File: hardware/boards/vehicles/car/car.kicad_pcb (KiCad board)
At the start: 2 copper layers, 50 x 95 mm, 119 parts, among them J1 Conn_01x04_Socket, J10 Conn_02x03_Odd_Even, J2 Conn_01x05_Socket, J3 Conn_01x05_Socket, J4 Conn_01x05_Socket, J5 Conn_01x02_Socket, J6 SMA, J7 02x04, J8 Conn_01x04_Socket, J9 Conn_02x05_Odd_Even, M1 Motor_DC, M2 Motor_DC, Q1 FQP27P06, Q10 AO3400A, Q11 2N3904, Q12 2N3904, Q2 AO3400A, Q3 FQP27P06, Q4 AO3400A, Q5 2N3904, Q6 2N3904, Q7 FQP27P06, Q8 AO3400A, Q9 FQP27P06, SW1 SW_Push, U1 ATmega328P-A, U4 TPS54302, U5 AMS1117-3.3, U7 NRF24L01, U8 RFX2401C, Y1 8MHz, Y3 16MHz

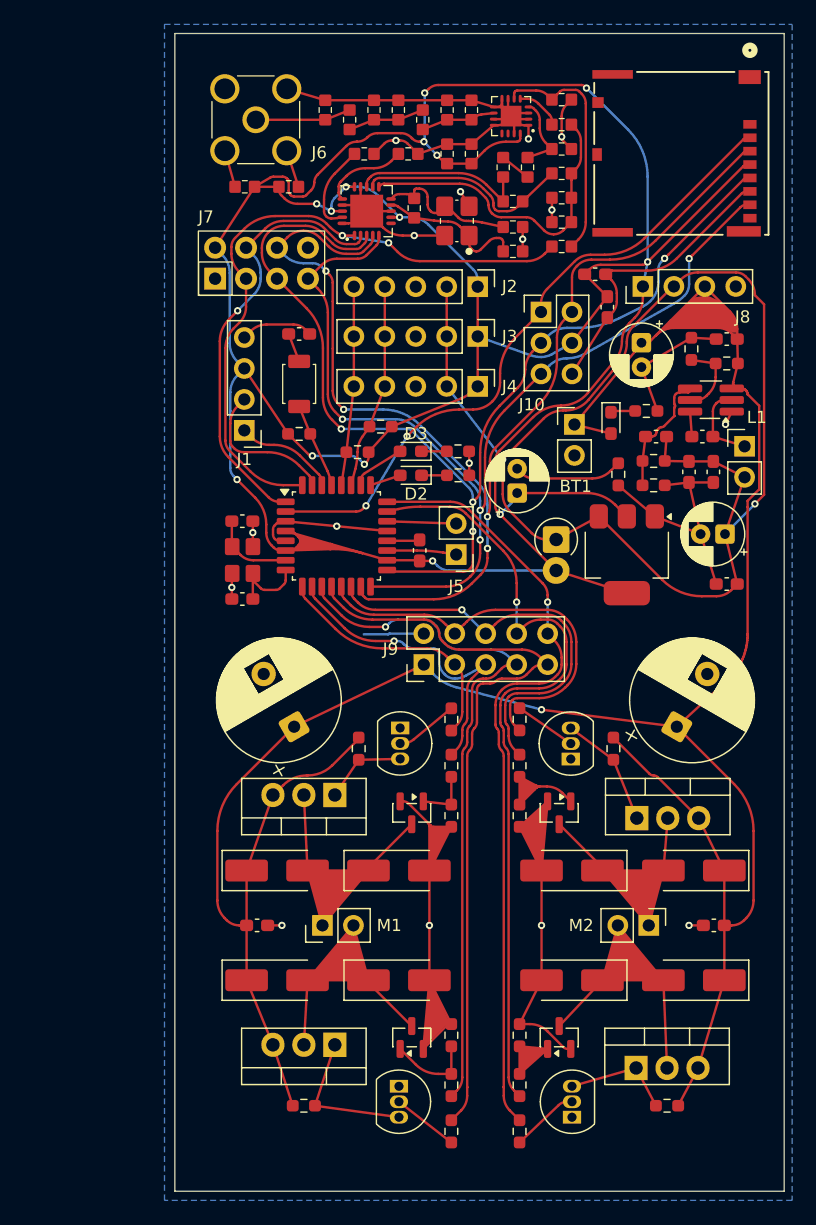
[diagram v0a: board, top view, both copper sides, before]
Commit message: REFACTO relinked every kicad projects
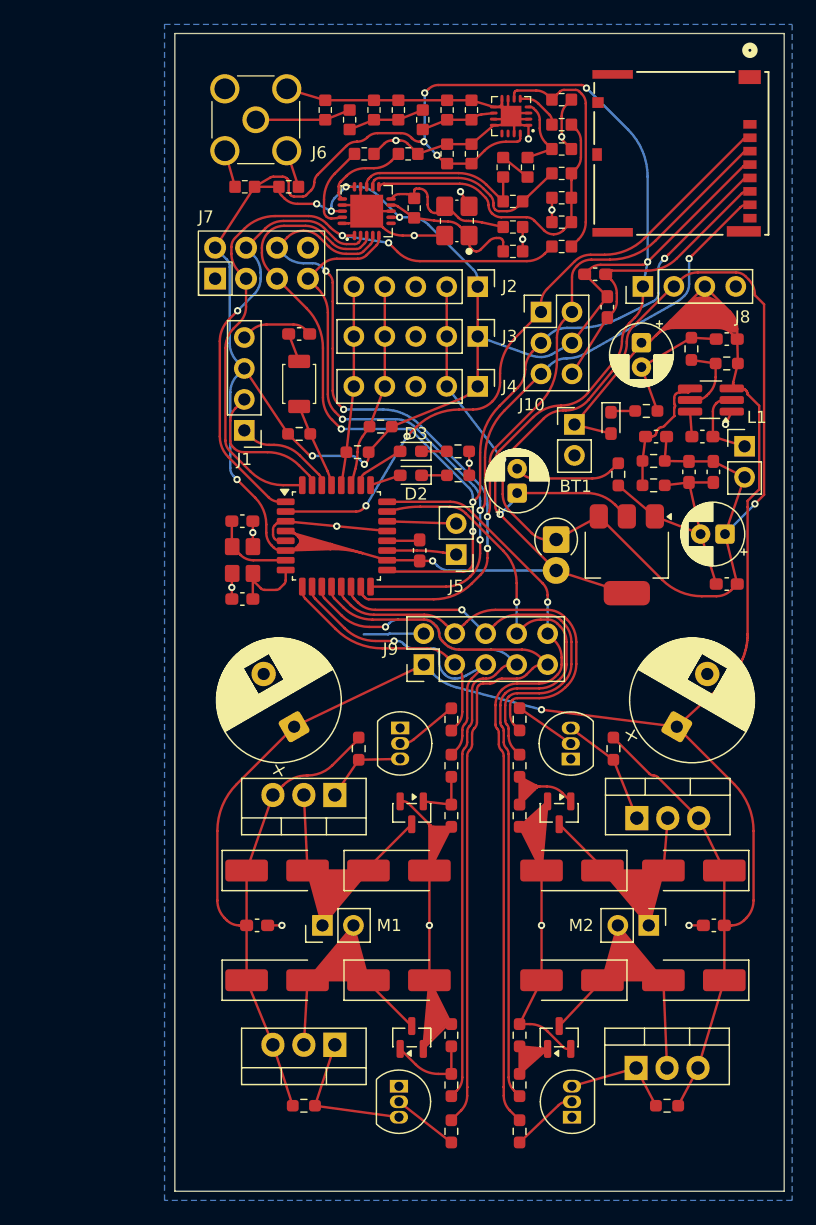
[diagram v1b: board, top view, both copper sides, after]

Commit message: car PCB
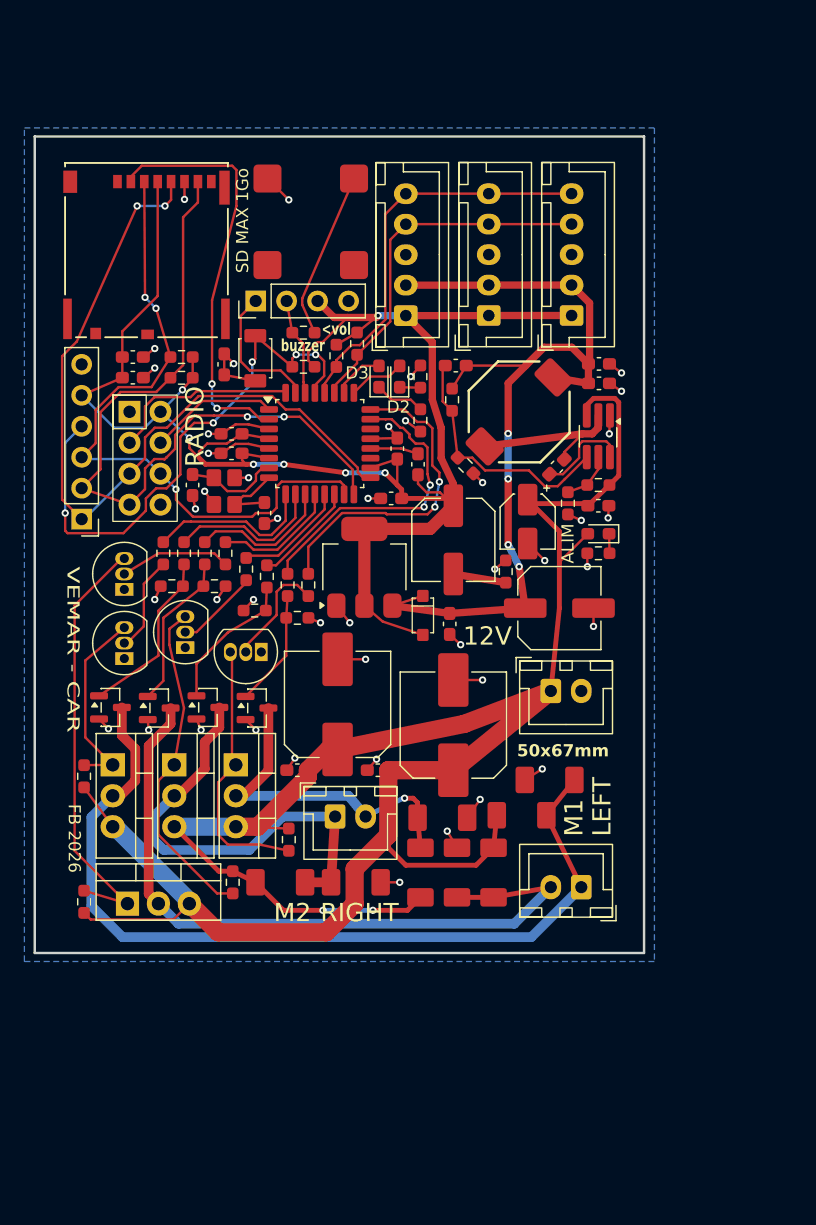
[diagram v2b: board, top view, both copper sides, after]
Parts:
- removed C24: 75pF, Capacitor_SMD:C_0603_1608Metric_Pad1.08x0.95mm_HandSolder
- removed C25: 10nF, common:C_0603
- removed C26: 1nF, common:C_0603
- removed C27: 33nF, common:C_0603
- removed C28, C29: 12pF, common:C_0603
- removed C30: 2.2nF, common:C_0603
- removed C31: 4.7nF, common:C_0603
- removed C32, C37, C38, C39, C40: 1.5pF, common:C_0603
- removed C33: 1.0pF, common:C_0603
- removed C34: 220pF, common:C_0603
- removed C35: 1uF, common:C_0603
- removed C36: 0.3pF, common:C_0603
- removed C41, C43: 22uF, Capacitor_THT:CP_Radial_D5.0mm_P2.00mm
- removed C42: 100nF, Capacitor_SMD:C_0603_1608Metric_Pad1.08x0.95mm_HandSolder
- removed J10: Conn_02x03_Odd_Even, Connector_PinHeader_2.54mm:PinHeader_2x03_P2.54mm_Vertical
- removed J7: 02x04, connector:Pin_02x04
- removed J8: Conn_01x04_Socket, Connector_PinHeader_2.54mm:PinHeader_1x04_P2.54mm_Vertical
- removed J9: Conn_02x05_Odd_Even, Connector_PinHeader_2.54mm:PinHeader_2x05_P2.54mm_Vertical
- removed L10, L9: 2.4nH, common:L_0603
- removed L6: 8.2nH, common:L_0603
- removed L7: 2.7nH, common:L_0603
- removed L8: 3.9nH, common:L_0603
- removed R31: 1, Resistor_SMD:R_0603_1608Metric_Pad0.98x0.95mm_HandSolder
- removed R32: 1M, common:R_0603
- removed U4: TPS54302, Package_TO_SOT_SMD:TSOT-23-6_HandSoldering
- removed U5: AMS1117-3.3, Package_TO_SOT_SMD:SOT-223-3_TabPin2
- removed U7: NRF24L01, transceiver:NRF24L01_QFN20
- removed U8: RFX2401C, transceiver:RFX2401C_QFN16
- removed Y3: 16MHz, common:Crystal_3225
- added BZ1: Buzzer, common:buzzer_8.5x8.5, F.Cu at (135.5, 69.7)
- added C10: 100nF, Capacitor_SMD:C_0603_1608Metric_Pad1.08x0.95mm_HandSolder, F.Cu at (159.1, 93.0)
- added C11: 100nF, Capacitor_SMD:C_0603_1608Metric_Pad1.08x0.95mm_HandSolder, F.Cu at (155.7, 89.8)
- added C12: 22uF, Capacitor_SMD:C_0603_1608Metric_Pad1.08x0.95mm_HandSolder, F.Cu at (159.2, 83.0)
- added C17: 22uF, common:CP_Elec_6.3x5.4, F.Cu at (147.2, 95.8)
- added C18: 100nF, Capacitor_SMD:C_0603_1608Metric_Pad1.08x0.95mm_HandSolder, F.Cu at (120.9, 82.5)
- added C7: 100nF, Capacitor_SMD:C_0603_1608Metric_Pad1.08x0.95mm_HandSolder, F.Cu at (142.6, 88.3)
- added C8: 100nF, Capacitor_SMD:C_0603_1608Metric_Pad1.08x0.95mm_HandSolder, F.Cu at (144.3, 89.6)
- added C9: 10uF, Capacitor_SMD:CP_Elec_4x5.4, F.Cu at (153.3, 94.3)
- added U2: TPS54302, Package_TO_SOT_SMD:TSOT-23-6_HandSoldering, F.Cu at (159.1, 87.3)
- added U3: AMS1117-3.3, Package_TO_SOT_SMD:SOT-223-3_TabPin2, F.Cu at (139.9, 98.0)
- BT1: value Battery 12V -> JST; footprint Connector_PinHeader_2.54mm:PinHeader_1x02_P2.54mm_Vertical -> Connector_JST:JST_XH_B2B-XH-A_1x02_P2.50mm_Vertical
- C13: value 470uF -> 22uF; footprint Capacitor_THT:CP_Radial_D10.0mm_P5.00mm -> Capacitor_SMD:C_0603_1608Metric_Pad1.08x0.95mm_HandSolder
- C14: value 100nF -> 75pF
- C15: value 470uF -> 22uF; footprint Capacitor_THT:CP_Radial_D10.0mm_P5.00mm -> common:CP_Elec_6.3x5.4
- C19: footprint Capacitor_THT:CP_Radial_D5.0mm_P2.00mm -> Capacitor_SMD:C_0603_1608Metric_Pad1.08x0.95mm_HandSolder
- C20: value 100nF -> 470uF; footprint Capacitor_SMD:C_0603_1608Metric_Pad1.08x0.95mm_HandSolder -> common:CP_Elec_8x10.5
- C22: value 22uF -> 470uF; footprint Capacitor_SMD:C_0603_1608Metric_Pad1.08x0.95mm_HandSolder -> common:CP_Elec_8x10.5
- C23: value 22uF -> 100nF
- C4: value 100nF -> 4.7uF
- C5: value 10uF -> 100nF
- D1, D3: value LED -> RED
- D10, D11, D5, D6, D7, D8, D9: footprint Diode_SMD:D_SMA_Handsoldering -> common:SMA(DO-214AC)
- D12: value 1N400x -> SS36; footprint Diode_THT:D_DO-41_SOD81_P2.54mm_Vertical_AnodeUp -> common:SMA(DO-214AC)
- D2: value LED -> GREEN
- D4: value SS36 -> RS1MFA; footprint Diode_SMD:D_SMA_Handsoldering -> common:D_SOD123
- J1: value Conn_01x04_Socket -> Dupont; footprint Connector_PinHeader_2.54mm:PinHeader_1x04_P2.54mm_Vertical -> Connector_PinHeader_2.54mm:PinHeader_1x06_P2.54mm_Vertical
- J2: value Conn_01x05_Socket -> Dupont; footprint Connector_PinHeader_2.54mm:PinHeader_1x05_P2.54mm_Vertical -> Connector_PinHeader_2.54mm:PinHeader_1x04_P2.54mm_Vertical
- J3: value Conn_01x05_Socket -> Dupont; footprint Connector_PinHeader_2.54mm:PinHeader_1x05_P2.54mm_Vertical -> connector:Pin_02x04
- J4: value Conn_01x05_Socket -> JST; footprint Connector_PinHeader_2.54mm:PinHeader_1x05_P2.54mm_Vertical -> Connector_JST:JST_XH_B5B-XH-A_1x05_P2.50mm_Vertical
- J5: value Conn_01x02_Socket -> JST; footprint Connector_PinHeader_2.54mm:PinHeader_1x02_P2.54mm_Vertical -> Connector_JST:JST_XH_B5B-XH-A_1x05_P2.50mm_Vertical
- J6: value SMA -> JST; footprint connector:SMA -> Connector_JST:JST_XH_B5B-XH-A_1x05_P2.50mm_Vertical
- L1: footprint Connector_PinHeader_2.54mm:PinHeader_1x02_P2.54mm_Vertical -> common:Inductor_octogone
- M1: value Motor_DC -> LEFT; footprint Connector_PinHeader_2.54mm:PinHeader_1x02_P2.54mm_Vertical -> Connector_JST:JST_XH_B2B-XH-A_1x02_P2.50mm_Vertical
- M2: value Motor_DC -> RIGHT; footprint Connector_PinHeader_2.54mm:PinHeader_1x02_P2.54mm_Vertical -> Connector_JST:JST_XH_B2B-XH-A_1x02_P2.50mm_Vertical
- Q2, Q8: value AO3400A -> FQP27P06; footprint Package_TO_SOT_SMD:SOT-23 -> Package_TO_SOT_THT:TO-220-3_Vertical
- Q3, Q9: value FQP27P06 -> AO3400A; footprint Package_TO_SOT_THT:TO-220-3_Vertical -> Package_TO_SOT_SMD:SOT-23
- R10: value 10K -> 43.2K
- R11: value 10K -> 5.76K
- R12: value 4.7K -> 1
- R13, R21: value 47 -> 10K
- R14, R22: value 1K -> 10K
- R16: value 47 -> 1K
- R17: value 4.7K -> 47
- R18: value 10K -> 47
- R19: value 10K -> 4.7K
- R23: value 511K -> 1K
- R24: value 22k -> 1K; footprint common:R_0603 -> Resistor_SMD:R_0603_1608Metric_Pad0.98x0.95mm_HandSolder
- R25: value 105K -> 47
- R26: value 1k -> 47; footprint common:R_0603 -> Resistor_SMD:R_0603_1608Metric_Pad0.98x0.95mm_HandSolder
- R27: value 1k -> 4.7K; footprint common:R_0603 -> Resistor_SMD:R_0603_1608Metric_Pad0.98x0.95mm_HandSolder
- R28: value 20k -> 4.7K; footprint common:R_0603 -> Resistor_SMD:R_0603_1608Metric_Pad0.98x0.95mm_HandSolder
- R29: value 43.2K -> 10K
- R30: value 5.76K -> 10K
- R5: value 4.7K -> ?
- R7: value 1K -> 4.7K
- R8: value 47 -> 511K
- R9: value 4.7K -> 105K
- SD1: value ~ -> SD Card Slot
- Y1: value 8MHz -> 16MHz
- moved R14 65.7 mm to (124.9, 82.5), turned to 180 degrees
- moved R28 64.7 mm to (133.7, 120.4), turned to -90 degrees
- moved R13 63.7 mm to (124.9, 80.8), turned to 180 degrees
- moved R27 58.7 mm to (129.1, 123.9), turned to 90 degrees
- moved R22 51.3 mm to (127.6, 99.6), turned to 180 degrees
- moved R20 50.7 mm to (116.9, 125.5), turned to 90 degrees
- moved R21 49.9 mm to (124.1, 99.6), turned to 180 degrees
- moved C14 48.7 mm to (147.4, 81.5)
- moved R12 46.9 mm to (151.5, 98.4), turned to -90 degrees
- moved R11 46.8 mm to (148.2, 89.7), turned to 135 degrees
- moved Q6 46.6 mm to (120.2, 99.9), turned to 90 degrees
- moved Q9 45.9 mm to (127.1, 109.5)
- moved Q12 45.9 mm to (131.4, 105.0), turned to 180 degrees
- moved SD1 44.6 mm to (122.0, 72.0), turned to 0 degrees
- moved R26 44.0 mm to (133.6, 99.5), turned to 90 degrees
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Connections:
- C1 pad 2: Net-(C1-Pad2) -> GND
- C13 pad 1: 12V -> GND
- C13 pad 2: GND -> 5V
- C14 pad 1: 12V -> Net-(U2-FB)
- C14 pad 2: GND -> 5V
- C15 pad 1: 12V -> 5V
- C16 pad 1: 12V -> GND
- C16 pad 2: GND -> 5V
- C19 pad 1: 12V -> 3V3
- C20 pad 1: GND -> 12V
- C20 pad 2: 12V -> GND
- C21 pad 1: Net-(U4-BOOT) -> 12V
- C21 pad 2: Net-(U4-SW) -> GND
- C22 pad 1: 5V -> 12V
- C23 pad 1: GND -> 12V
- C23 pad 2: 5V -> GND
- C4 pad 2: Net-(U1-AREF) -> GND
- D10 pad 1: 12V -> Net-(D10-K)
- D10 pad 2: Net-(D10-A) -> GND
- D11 pad 1: Net-(D10-A) -> 12V
- D11 pad 2: GND -> Net-(D11-A)
- D12 pad 1: 5V -> Net-(D11-A)
- D12 pad 2: 3V3 -> GND
- D4 pad 1: 12V -> 5V
- D4 pad 2: Net-(D4-A) -> 3V3
- D5 pad 1: Net-(D4-A) -> 12V
- D5 pad 2: GND -> Net-(D5-A)
- D6 pad 1: 12V -> Net-(D5-A)
- D6 pad 2: Net-(D6-A) -> GND
- D7 pad 1: Net-(D6-A) -> 12V
- D7 pad 2: GND -> Net-(D7-A)
- D8 pad 1: 12V -> Net-(D7-A)
- D8 pad 2: Net-(D8-A) -> GND
- D9 pad 1: Net-(D8-A) -> 12V
- D9 pad 2: GND -> Net-(D10-K)
- J1 pad 1: RX -> SCK
- J1 pad 2: TX -> MISO
- J1 pad 3: 3V3 -> MOSI
- J1 pad 4: GND -> RST
- J2 pad 1: 3V3 -> TX
- J2 pad 2: 5V -> RX
- J2 pad 3: GND -> 3V3
- J2 pad 4: SDA -> GND
- J3 pad 1: 3V3 -> GND
- J3 pad 2: 5V -> RC_EN
- J3 pad 3: GND -> SCK
- J3 pad 4: SDA -> MISO
- J3 pad 5: SCL -> unconnected-(J3-Pad5)
- J5 pad 1: ADC0 -> 3V3
- J5 pad 2: ADC1 -> 5V
- J6 pad 1: Net-(J6-ANT) -> 3V3
- J6 pad 2: GND -> 5V
- J6 pad 4: GND -> SDA
- J6 pad 5: GND -> SCL
- L1 pad 1: Net-(U4-SW) -> Net-(U2-SW)
- M1 pad 1: Net-(D4-A) -> Net-(D5-A)
- M1 pad 2: Net-(D6-A) -> Net-(D7-A)
- M2 pad 1: Net-(D8-A) -> Net-(D10-K)
- M2 pad 2: Net-(D10-A) -> Net-(D11-A)
- Q1 pad 2: Net-(D4-A) -> Net-(D5-A)
- Q10 pad 3: Net-(D10-A) -> Net-(D11-A)
- Q2 pad 2: GND -> Net-(D7-A)
- Q2 pad 3: Net-(D4-A) -> 12V
- Q3 pad 2: Net-(D6-A) -> GND
- Q3 pad 3: 12V -> Net-(D5-A)
- Q4 pad 3: Net-(D6-A) -> Net-(D7-A)
- Q6 pad 3: Net-(Q3-G) -> Net-(Q2-G)
- Q7 pad 2: Net-(D8-A) -> Net-(D10-K)
- Q8 pad 1: Net-(Q8-G) -> Net-(Q12-C)
- Q8 pad 2: GND -> Net-(D11-A)
- Q8 pad 3: Net-(D8-A) -> 12V
- Q9 pad 1: Net-(Q12-C) -> Net-(Q9-G)
- Q9 pad 2: Net-(D10-A) -> GND
- Q9 pad 3: 12V -> Net-(D10-K)
- R10 pad 1: Net-(Q2-G) -> Net-(U2-FB)
- R10 pad 2: GND -> 5V
- R11 pad 2: Net-(Q4-G) -> Net-(U2-FB)
- R12 pad 1: 12V -> GND
- R12 pad 2: Net-(Q3-G) -> Net-(C17-Pad2)
- R13 pad 1: Net-(Q4-G) -> 3V3
- R13 pad 2: M1_EN_CW -> MOSI
- R14 pad 1: M1_EN_CCW -> 3V3
- R14 pad 2: Net-(Q6-B) -> MISO
- R15 pad 1: M2_PWM_CW -> M1_PWM_CW
- R15 pad 2: Net-(Q11-B) -> Net-(Q5-B)
- R16 pad 1: Net-(Q8-G) -> M1_EN_CCW
- R16 pad 2: M2_PWM_CCW -> Net-(Q6-B)
- R17 pad 1: Net-(Q11-C) -> Net-(Q3-G)
- R17 pad 2: 12V -> M1_PWM_CCW
- R18 pad 1: Net-(Q8-G) -> Net-(Q4-G)
- R18 pad 2: GND -> M1_EN_CW
- R19 pad 1: GND -> Net-(Q1-G)
- R19 pad 2: Net-(Q10-G) -> 12V
- R20 pad 2: Net-(Q12-C) -> Net-(Q2-G)
- R21 pad 1: Net-(Q10-G) -> Net-(Q3-G)
- R21 pad 2: M2_EN_CW -> GND
- R22 pad 1: M2_EN_CCW -> GND
- R22 pad 2: Net-(Q12-B) -> Net-(Q4-G)
- R23 pad 1: Net-(U4-EN) -> M2_PWM_CW
- R23 pad 2: 12V -> Net-(Q11-B)
- R24 pad 1: GND -> M2_EN_CCW
- R24 pad 2: Net-(U7-IREF) -> Net-(Q12-B)
- R25 pad 1: GND -> Net-(Q9-G)
- R25 pad 2: Net-(U4-EN) -> M2_PWM_CCW
- R26 pad 1: Net-(U7-VDD_PA) -> Net-(Q10-G)
- R26 pad 2: Net-(U8-TXEN) -> M2_EN_CW
- R27 pad 1: RC_EN -> Net-(Q11-C)
- R27 pad 2: Net-(U8-RXEN) -> 12V
- R28 pad 1: GND -> 12V
- R28 pad 2: Net-(U8-RXEN) -> Net-(Q12-C)
- R29 pad 1: Net-(U4-FB) -> Net-(Q9-G)
- R29 pad 2: 5V -> GND
- R30 pad 2: Net-(U4-FB) -> Net-(Q10-G)
- R5 pad 1: 3V3 -> RX
- R5 pad 2: SDA -> Net-(BZ1-Pad1)
- R6 pad 2: SCL -> SDA
- R7 pad 1: M1_PWM_CW -> 3V3
- R7 pad 2: Net-(Q5-B) -> SCL
- R8 pad 1: Net-(Q2-G) -> Net-(U2-EN)
- R8 pad 2: M1_PWM_CCW -> 12V
- R9 pad 1: Net-(Q1-G) -> GND
- R9 pad 2: 12V -> Net-(U2-EN)
- SW1 pad 1: Net-(C1-Pad2) -> GND
- U1 pad 19: ADC0 -> unconnected-(U1-ADC6-Pad19)
- U1 pad 22: ADC1 -> unconnected-(U1-ADC7-Pad22)
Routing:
- net GND: track 229.7 -> 72.8 mm, vias 16 -> 43
- net 3V3: track 271.7 -> 149.5 mm, vias 14 -> 7
- net Net-(D5-A): track 0.00 -> 71.8 mm
- net Net-(D7-A): track 0.00 -> 59.0 mm
- net M1_EN_CCW: track 62.8 -> 10.3 mm
- net M1_EN_CW: track 57.8 -> 11.8 mm, vias 1 -> 0
- net MOSI: track 99.5 -> 54.7 mm, vias 4 -> 3
- net M2_EN_CW: track 65.2 -> 25.0 mm, vias 1 -> 2
- net RST: track 7.00 -> 46.9 mm, vias 0 -> 5
- net RC_EN: track 54.5 -> 15.6 mm, vias 2 -> 0
- net 5V: track 111.1 -> 73.0 mm, vias 2 -> 4
- net M2_EN_CCW: track 64.5 -> 26.5 mm, vias 1 -> 2
- net Net-(D10-K): track 0.00 -> 37.2 mm
- net 12V: track 211.6 -> 180.1 mm, vias 1 -> 2
- net Net-(Q2-G): track 4.60 -> 35.7 mm
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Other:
- board size 50 x 95 mm -> 50 x 67 mm
- board text added: "12V"
- board text added: "50x67mm"
- board text added: "<vol"
- board text added: "ALIM"
- board text added: "FB 2026"
- board text added: "I2C"
- board text added: "RADIO"
- board text added: "SD MAX 1Go"
- board text added: "SPI"
- board text added: "UART"
- board text added: "VEMAR - CAR"
- board text added: "buzzer"
- board text removed: "D4"
